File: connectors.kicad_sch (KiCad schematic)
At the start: 18 parts, among them J2 Conn_WS2812_Extern, T7 AO3400A, T8 AO3400A, X10 S4B-PH-SM4-K-TB(LF)(SN), X13 KF2EDGR-3.81-3P, X5 KF2EDGR-3.81-3P, X7 BH-00105, X8 USB3.1C16PFSMT

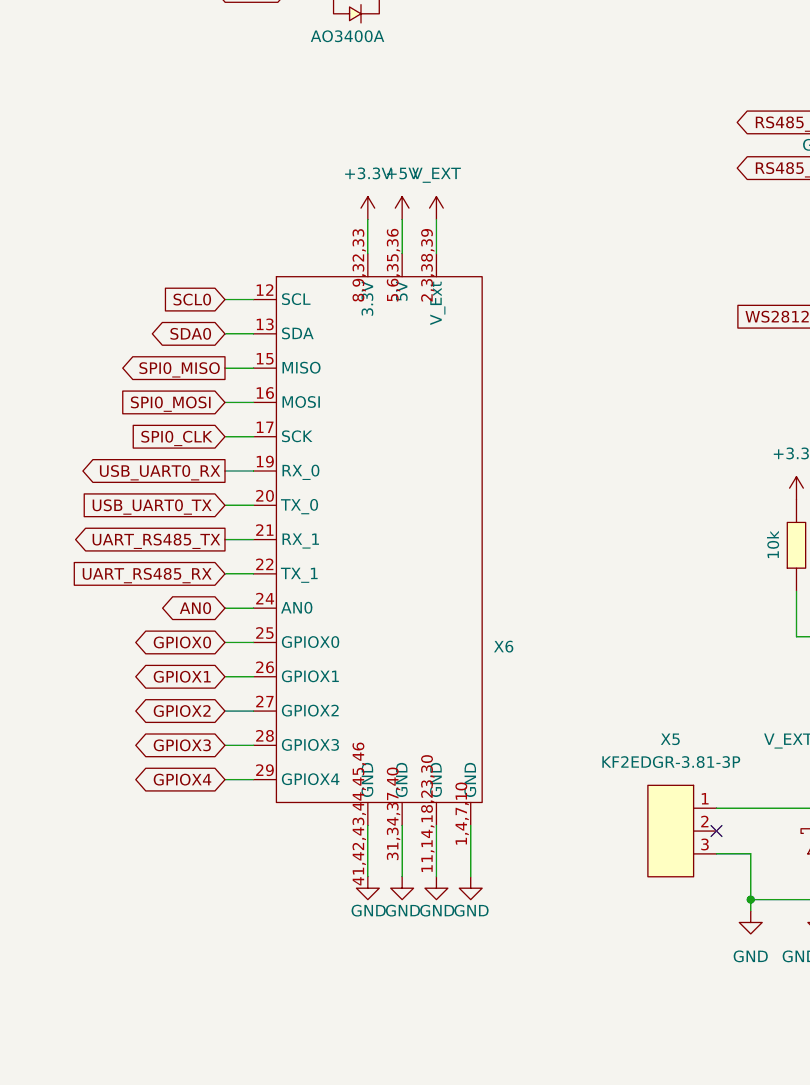
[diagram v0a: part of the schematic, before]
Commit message: Layout of parts done. Started laying tracks
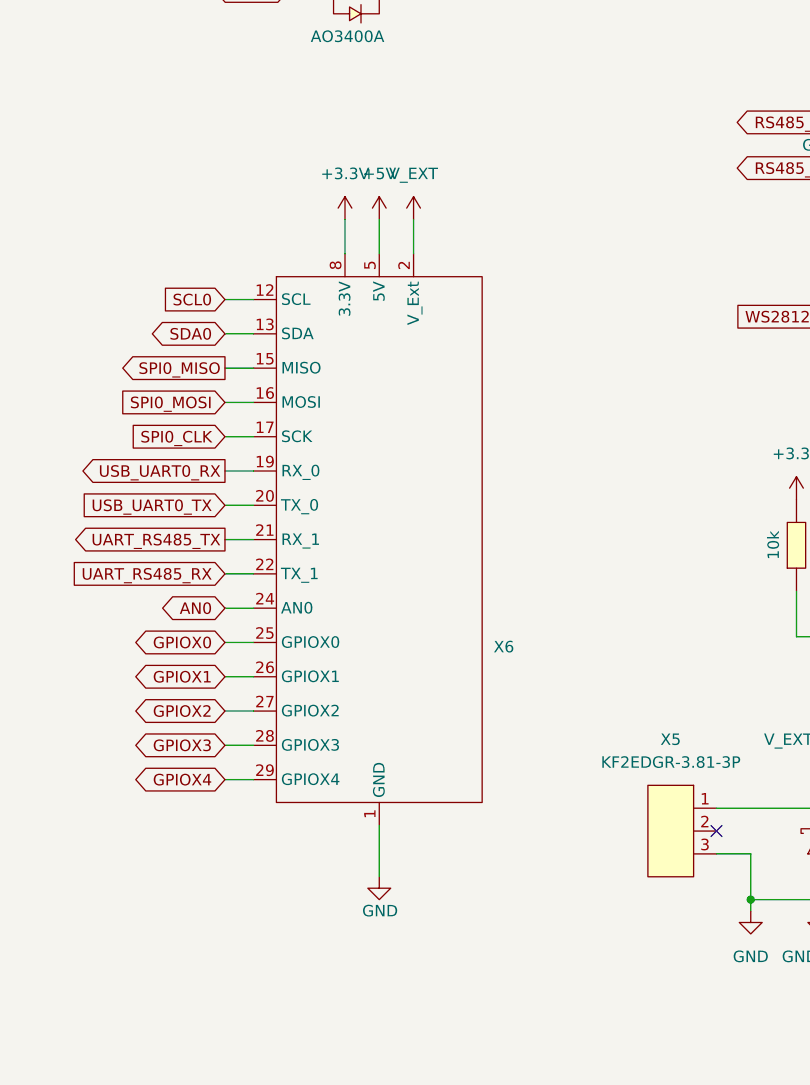
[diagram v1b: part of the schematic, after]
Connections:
- net +3.3V: now also X6.32 (3.3V), X6.33 (3.3V), X6.8 (3.3V), X6.9 (3.3V); no longer X6.8,9,32,33 (3.3V)
- net +5V: now also X6.35 (5V), X6.36 (5V), X6.5 (5V), X6.6 (5V); no longer X6.5,6,35,36 (5V)
- net GND: now also X6.1 (GND), X6.10 (GND), X6.11 (GND), X6.14 (GND), X6.18 (GND), X6.23 (GND), X6.30 (GND), X6.31 (GND), X6.34 (GND), X6.37 (GND), X6.4 (GND), X6.40 (GND), X6.41 (GND), X6.42 (GND), X6.43 (GND), X6.44 (GND), X6.45 (GND), X6.46 (GND), X6.7 (GND); no longer X6.1,4,7,10 (GND), X6.11,14,18,23,30 (GND), X6.31,34,37,40 (GND), X6.41,42,43,44,45,46 (GND)
- net V_EXT: now also X6.2 (V_Ext), X6.3 (V_Ext), X6.38 (V_Ext), X6.39 (V_Ext); no longer X6.2,3,38,39 (V_Ext)
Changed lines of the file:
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@@
     (stroke (width 0) (type default))
   )
-  (wire (pts (xy 195.58 77.47) (xy 195.58 81.28))
+  (wire (pts (xy 193.04 77.47) (xy 193.04 81.28))
     (stroke (width 0) (type default))
   )
@@
     (stroke (width 0) (type default))
   )
-  (wire (pts (xy 191.77 77.47) (xy 191.77 81.28))
+  (wire (pts (xy 189.23 77.47) (xy 189.23 81.28))
     (stroke (width 0) (type default))
   )
@@
     (stroke (width 0) (type default))
   )
-  (wire (pts (xy 203.2 144.78) (xy 203.2 150.495))
-    (stroke (width 0) (type default))
-  )
   (wire (pts (xy 213.36 30.48) (xy 213.36 52.07))
     (stroke (width 0) (type default))
@@
     (stroke (width 0) (type default))
   )
-  (wire (pts (xy 199.39 144.78) (xy 199.39 150.495))
-    (stroke (width 0) (type default))
-  )
   (wire (pts (xy 61.595 80.645) (xy 61.595 98.425))
     (stroke (width 0) (type default))
@@
     (stroke (width 0) (type default))
   )
-  (wire (pts (xy 195.58 144.78) (xy 195.58 150.495))
-    (stroke (width 0) (type default))
-  )
-  (wire (pts (xy 191.77 144.78) (xy 191.77 150.495))
-    (stroke (width 0) (type default))
-  )
-  (wire (pts (xy 199.39 77.47) (xy 199.39 81.28))
+  (wire (pts (xy 193.04 144.78) (xy 193.04 150.495))
+    (stroke (width 0) (type default))
+  )
+  (wire (pts (xy 196.85 77.47) (xy 196.85 81.28))
     (stroke (width 0) (type default))
   )
@@
         (path "/280adf03-05ea-4001-ab24-a5a43e6d4cc9/bbe51f60-6efe-4402-8542-2dfbd71b2c52"
           (reference "X13") (unit 1)
-        )
-      )
-    )
-  )
-  (symbol (lib_id "eduboardv2:GND") (at 203.2 150.495 0) (unit 1)
-    (in_bom yes) (on_board yes) (dnp no)
-    (property "Reference" "#PWR0102" (at 203.2 156.845 0)
-      (effects (font (size 1.27 1.27)) hide)
-    )
-    (property "Value" "GND" (at 201.295 154.305 0)
-      (effects (font (size 1.27 1.27)) (justify left))
-    )
-    (property "Footprint" "" (at 203.2 150.495 0)
-      (effects (font (size 1.27 1.27)) hide)
-    )
-    (property "Datasheet" "" (at 203.2 150.495 0)
-      (effects (font (size 1.27 1.27)) hide)
-    )
-    (pin "1")
-    (instances
-      (project "EduboardV2_Baseboard"
-        (path "/280adf03-05ea-4001-ab24-a5a43e6d4cc9/bbe51f60-6efe-4402-8542-2dfbd71b2c52"
-          (reference "#PWR0102") (unit 1)
         )
       )
@@
       (effects (font (size 1.27 1.27)) hide)
     )
-    (pin "1,4,7,10")
-    (pin "11,14,18,23,30")
+    (pin "1")
+    (pin "10")
+    (pin "11")
     (pin "12")
     (pin "13")
+    (pin "14")
     (pin "15")
     (pin "16")
     (pin "17")
+    (pin "18")
     (pin "19")
-    (pin "2,3,38,39")
+    (pin "2")
     (pin "20")
     (pin "21")
     (pin "22")
+    (pin "23")
     (pin "24")
     (pin "25")
@@
     (pin "28")
     (pin "29")
-    (pin "31,34,37,40")
-    (pin "41,42,43,44,45,46")
-    (pin "5,6,35,36")
-    (pin "8,9,32,33")
+    (pin "3")
+    (pin "30")
+    (pin "31")
+    (pin "32")
+    (pin "33")
+    (pin "34")
+    (pin "35")
+    (pin "36")
+    (pin "37")
+    (pin "38")
+    (pin "39")
+    (pin "4")
+    (pin "40")
+    (pin "41")
+    (pin "42")
+    (pin "43")
+    (pin "44")
+    (pin "45")
+    (pin "46")
+    (pin "5")
+    (pin "6")
+    (pin "7")
+    (pin "8")
+    (pin "9")
     (instances
       (project "EduboardV2_Baseboard"
@@
     )
   )
-  (symbol (lib_id "eduboardv2:GND") (at 199.39 150.495 0) (unit 1)
-    (in_bom yes) (on_board yes) (dnp no)
-    (property "Reference" "#PWR0101" (at 199.39 156.845 0)
-      (effects (font (size 1.27 1.27)) hide)
-    )
-    (property "Value" "GND" (at 197.485 154.305 0)
-      (effects (font (size 1.27 1.27)) (justify left))
-    )
-    (property "Footprint" "" (at 199.39 150.495 0)
-      (effects (font (size 1.27 1.27)) hide)
-    )
-    (property "Datasheet" "" (at 199.39 150.495 0)
-      (effects (font (size 1.27 1.27)) hide)
-    )
-    (pin "1")
-    (instances
-      (project "EduboardV2_Baseboard"
-        (path "/280adf03-05ea-4001-ab24-a5a43e6d4cc9/bbe51f60-6efe-4402-8542-2dfbd71b2c52"
-          (reference "#PWR0101") (unit 1)
-        )
-      )
-    )
-  )
   (symbol (lib_id "eduboardv2:GND") (at 41.275 101.6 0) (unit 1)
     (in_bom yes) (on_board yes) (dnp no) (fields_autoplaced)
@@
     )
   )
-  (symbol (lib_name "V_EXT_1") (lib_id "eduboardv2:V_EXT") (at 199.39 77.47 0) (unit 1)
-    (in_bom yes) (on_board yes) (dnp no) (fields_autoplaced)
-    (property "Reference" "#PWR017" (at 199.39 81.28 0)
-      (effects (font (size 1.27 1.27)) hide)
-    )
-    (property "Value" "V_EXT" (at 199.39 72.39 0)
-      (effects (font (size 1.27 1.27)))
-    )
-    (property "Footprint" "" (at 199.39 77.47 0)
-      (effects (font (size 1.27 1.27)) hide)
-    )
-    (property "Datasheet" "" (at 199.39 77.47 0)
+  (symbol (lib_name "V_EXT_1") (lib_id "eduboardv2:V_EXT") (at 196.85 77.47 0) (unit 1)
+    (in_bom yes) (on_board yes) (dnp no) (fields_autoplaced)
+    (property "Reference" "#PWR017" (at 196.85 81.28 0)
+      (effects (font (size 1.27 1.27)) hide)
+    )
+    (property "Value" "V_EXT" (at 196.85 72.39 0)
+      (effects (font (size 1.27 1.27)))
+    )
+    (property "Footprint" "" (at 196.85 77.47 0)
+      (effects (font (size 1.27 1.27)) hide)
+    )
+    (property "Datasheet" "" (at 196.85 77.47 0)
       (effects (font (size 1.27 1.27)) hide)
     )
@@
     )
   )
-  (symbol (lib_id "eduboardv2:GND") (at 191.77 150.495 0) (unit 1)
+  (symbol (lib_id "eduboardv2:GND") (at 193.04 150.495 0) (unit 1)
     (in_bom yes) (on_board yes) (dnp no)
-    (property "Reference" "#PWR098" (at 191.77 156.845 0)
-      (effects (font (size 1.27 1.27)) hide)
-    )
-    (property "Value" "GND" (at 189.865 154.305 0)
+    (property "Reference" "#PWR098" (at 193.04 156.845 0)
+      (effects (font (size 1.27 1.27)) hide)
+    )
+    (property "Value" "GND" (at 191.135 154.305 0)
       (effects (font (size 1.27 1.27)) (justify left))
     )
-    (property "Footprint" "" (at 191.77 150.495 0)
-      (effects (font (size 1.27 1.27)) hide)
-    )
-    (property "Datasheet" "" (at 191.77 150.495 0)
+    (property "Footprint" "" (at 193.04 150.495 0)
+      (effects (font (size 1.27 1.27)) hide)
+    )
+    (property "Datasheet" "" (at 193.04 150.495 0)
       (effects (font (size 1.27 1.27)) hide)
     )
@@
         (path "/280adf03-05ea-4001-ab24-a5a43e6d4cc9/bbe51f60-6efe-4402-8542-2dfbd71b2c52"
           (reference "#PWR098") (unit 1)
-        )
-      )
-    )
-  )
-  (symbol (lib_id "eduboardv2:GND") (at 195.58 150.495 0) (unit 1)
-    (in_bom yes) (on_board yes) (dnp no)
-    (property "Reference" "#PWR0100" (at 195.58 156.845 0)
-      (effects (font (size 1.27 1.27)) hide)
-    )
-    (property "Value" "GND" (at 193.675 154.305 0)
-      (effects (font (size 1.27 1.27)) (justify left))
-    )
-    (property "Footprint" "" (at 195.58 150.495 0)
-      (effects (font (size 1.27 1.27)) hide)
-    )
-    (property "Datasheet" "" (at 195.58 150.495 0)
-      (effects (font (size 1.27 1.27)) hide)
-    )
-    (pin "1")
-    (instances
-      (project "EduboardV2_Baseboard"
-        (path "/280adf03-05ea-4001-ab24-a5a43e6d4cc9/bbe51f60-6efe-4402-8542-2dfbd71b2c52"
-          (reference "#PWR0100") (unit 1)
         )
       )
@@
     )
   )
-  (symbol (lib_id "eduboardv2:+5V") (at 195.58 77.47 0) (unit 1)
-    (in_bom yes) (on_board yes) (dnp no) (fields_autoplaced)
-    (property "Reference" "#PWR096" (at 195.58 81.28 0)
-      (effects (font (size 1.27 1.27)) hide)
-    )
-    (property "Value" "+5V" (at 195.58 72.39 0)
-      (effects (font (size 1.27 1.27)))
-    )
-    (property "Footprint" "" (at 195.58 77.47 0)
-      (effects (font (size 1.27 1.27)) hide)
-    )
-    (property "Datasheet" "" (at 195.58 77.47 0)
+  (symbol (lib_id "eduboardv2:+5V") (at 193.04 77.47 0) (unit 1)
+    (in_bom yes) (on_board yes) (dnp no) (fields_autoplaced)
+    (property "Reference" "#PWR096" (at 193.04 81.28 0)
+      (effects (font (size 1.27 1.27)) hide)
+    )
+    (property "Value" "+5V" (at 193.04 72.39 0)
+      (effects (font (size 1.27 1.27)))
+    )
+    (property "Footprint" "" (at 193.04 77.47 0)
+      (effects (font (size 1.27 1.27)) hide)
+    )
+    (property "Datasheet" "" (at 193.04 77.47 0)
       (effects (font (size 1.27 1.27)) hide)
     )
@@
     )
   )
-  (symbol (lib_id "eduboardv2:+3.3V") (at 191.77 77.47 0) (unit 1)
-    (in_bom yes) (on_board yes) (dnp no) (fields_autoplaced)
-    (property "Reference" "#PWR01" (at 191.77 81.28 0)
-      (effects (font (size 1.27 1.27)) hide)
-    )
-    (property "Value" "+3.3V" (at 191.77 72.39 0)
-      (effects (font (size 1.27 1.27)))
-    )
-    (property "Footprint" "" (at 191.77 77.47 0)
-      (effects (font (size 1.27 1.27)) hide)
-    )
-    (property "Datasheet" "" (at 191.77 77.47 0)
-      (effects (font (size 1.27 1.27)) hide)
-    )
+  (symbol (lib_id "eduboardv2:+3.3V") (at 189.23 77.47 0) (unit 1)
+    (in_bom yes) (on_board yes) (dnp no) (fields_autoplaced)
+    (property "Reference" "#PWR01" (at 189.23 81.28 0)
+      (effects (font (size 1.27 1.27)) hide)
+    )
+    (property "Value" "+3.3V" (at 189.23 72.39 0)
+      (effects (font (size 1.27 1.27)))
+    )
+    (property "Footprint" "" (at 189.23 77.47 0)
+      (effects (font (size 1.27 1.27)) hide)
+    )
+    (property "Datasheet" "" (at 189.23 77.47 0)
+      (effects (font (size 1.27 1.27)) hide)
+    )

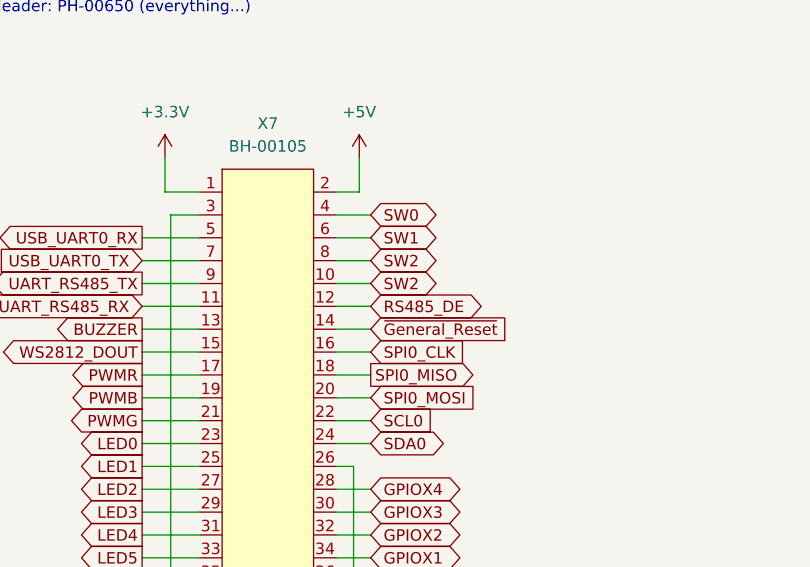
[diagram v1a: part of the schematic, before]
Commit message: proceed with layout
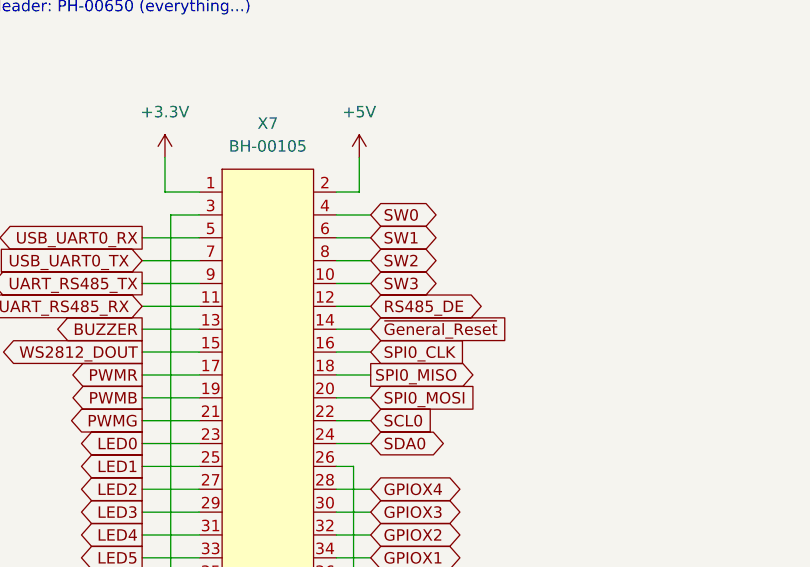
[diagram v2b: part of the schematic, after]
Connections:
- net SW2: no longer X7.10
- new net SW3: X7.10
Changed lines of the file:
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@@
     )
   )
-  (global_label "SW2" (shape bidirectional) (at 63.5 60.325 0) (fields_autoplaced)
+  (global_label "SW3" (shape bidirectional) (at 63.5 60.325 0) (fields_autoplaced)
     (effects (font (size 1.27 1.27)) (justify left))
     (property "Intersheetrefs" "${INTERSHEET_REFS}" (at 71.3875 60.325 0)
@@
   )
   (symbol (lib_id "eduboardv2:BH-00105") (at 52.07 70.485 0) (unit 1)
-    (in_bom yes) (on_board yes) (dnp no) (fields_autoplaced)
+    (in_bom yes) (on_board yes) (dnp no)
     (property "Reference" "X7" (at 52.07 42.545 0)
       (effects (font (size 1.27 1.27)))
